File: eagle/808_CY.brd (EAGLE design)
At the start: 100 x 80 mm, 112 parts, among them IC1 TL071P, IC2 TL071P, IC3 TL071P, IC4 TL072P, Q1 2N3904, Q2 2N3904, Q3 2N3904, Q4 2N3904, Q5 2N3904, Q6 2N3904, Q7 2N3904, Q8 2N3906

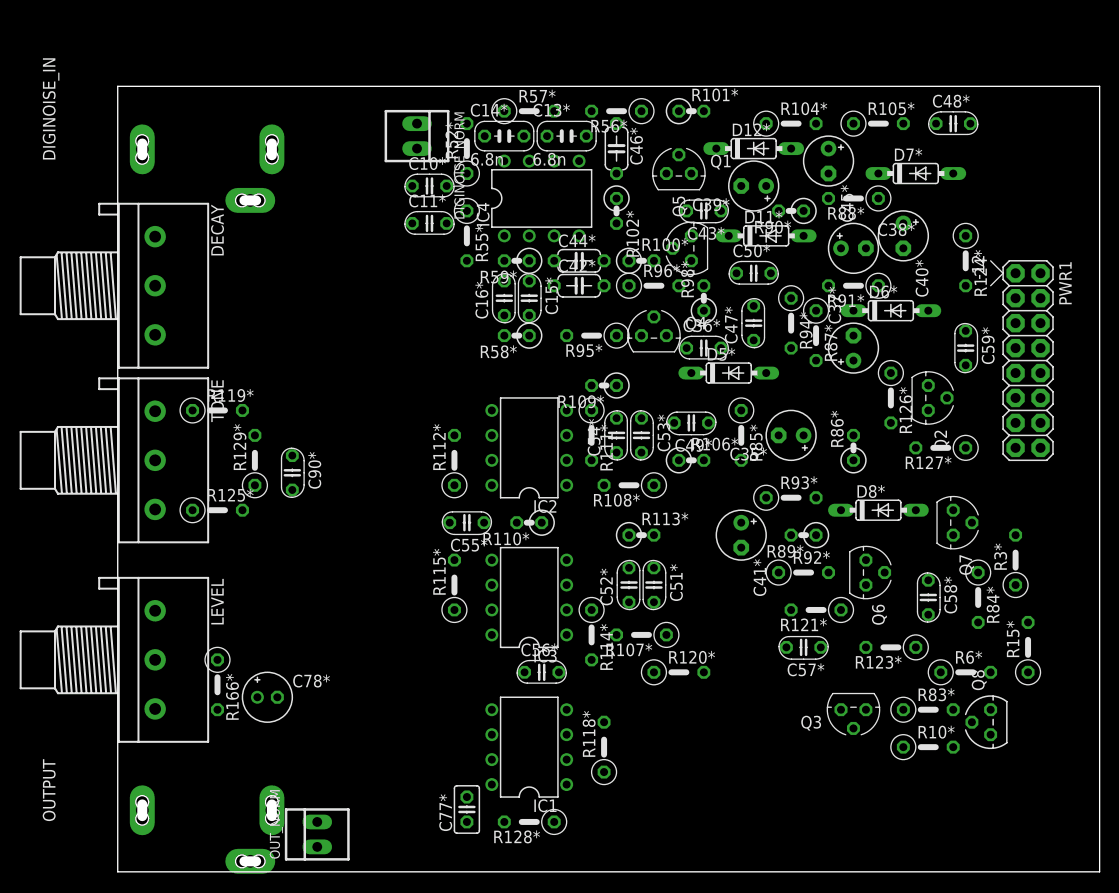
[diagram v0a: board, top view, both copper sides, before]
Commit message: 90 pct routed
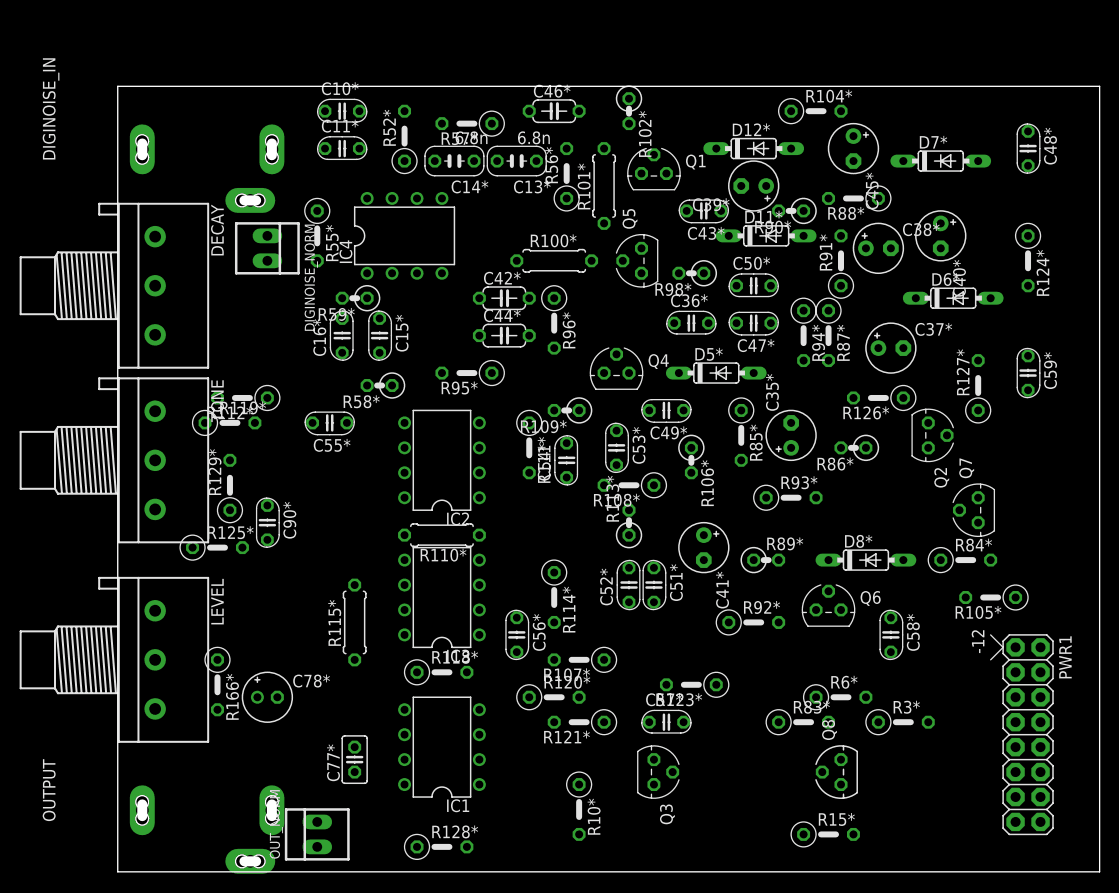
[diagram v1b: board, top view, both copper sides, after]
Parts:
- R100*, R101*, R110*: device TR808clone:0207/2V -> TR808clone:0207/7
- R115*: device TR808clone:0207/5V -> TR808clone:0207/7
- moved R105* 49.6 mm to (88.9, 27.9), turned to 180 degrees
- moved PWR1 38.1 mm to (92.7, 16.5)
- moved R10* 36.1 mm to (47.0, 6.35), turned to 270 degrees
- moved R15* 27.9 mm to (72.4, 3.81), turned to 0 degrees
- moved R121* 26.7 mm to (47.0, 15.2)
- moved R112* 22.5 mm to (12.7, 48.3), turned to 180 degrees
- moved Q3 21.3 mm to (54.6, 10.2), turned to 270 degrees
- moved R123* 20.7 mm to (58.4, 19.1)
- moved R3* 20.1 mm to (80.0, 15.2), turned to 0 degrees
- moved DIGINOISE_NORM 19.1 mm to (15.2, 63.5)
- moved R118* 18.2 mm to (33.0, 20.3), turned to 0 degrees
- moved C55* 17.3 mm to (21.6, 45.7)
- moved C16* 16.9 mm to (22.9, 54.6)
- moved R59* 16.9 mm to (24.1, 58.4)
- moved Q8 16.1 mm to (73.7, 10.2)
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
